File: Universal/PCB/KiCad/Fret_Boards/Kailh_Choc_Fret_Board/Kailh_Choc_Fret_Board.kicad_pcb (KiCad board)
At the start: 2 copper layers, 121 x 29 mm, 24 parts

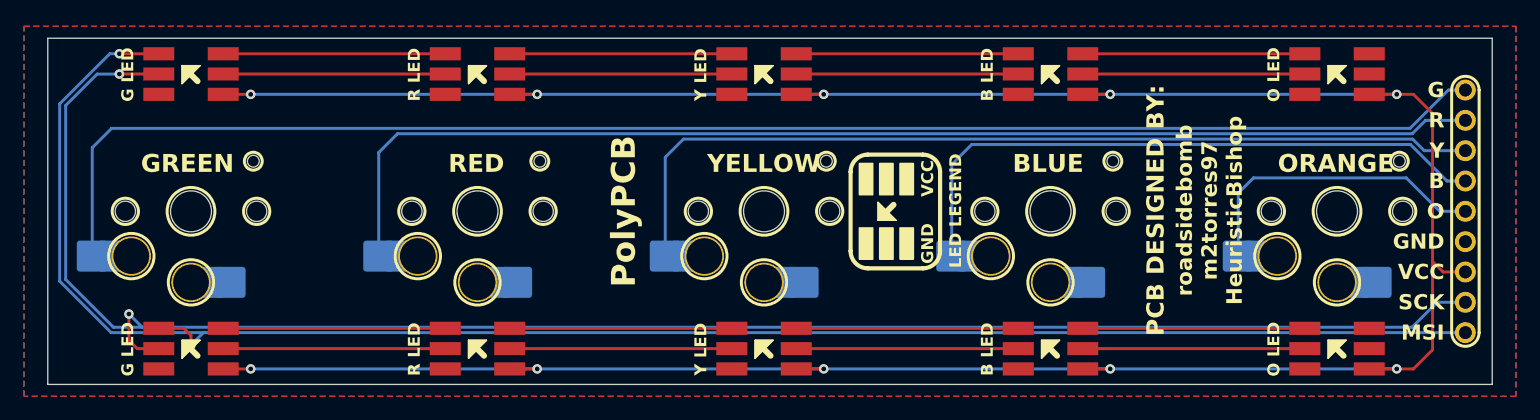
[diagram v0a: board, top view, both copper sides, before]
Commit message: updated The choc fret board
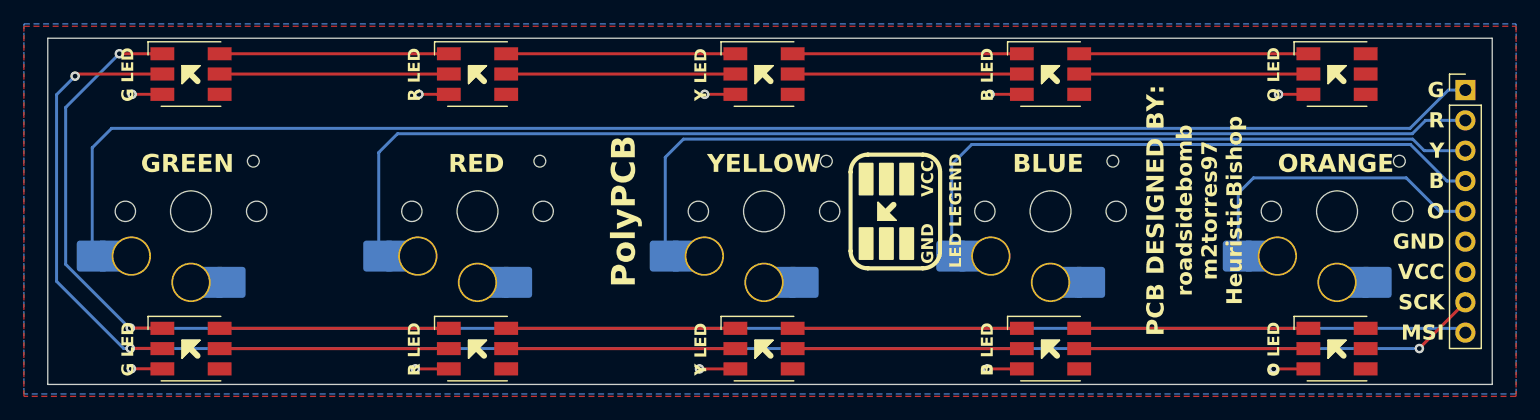
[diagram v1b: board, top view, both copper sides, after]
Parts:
- removed ? (x9): , 
- added J1: Conn_01x09_Pin, Connector_PinHeader_2.54mm:PinHeader_1x09_P2.54mm_Vertical, F.Cu at (180.8, 79.8)
- L1, U1: renamed from D1; footprint Controller_Inputs:LED_RGB_5050_DOTSTAR -> LED_SMD:LED_RGB_5050-6
- L2, U2: renamed from D2; footprint Controller_Inputs:LED_RGB_5050_DOTSTAR -> LED_SMD:LED_RGB_5050-6
- L3, U3: renamed from D3; footprint Controller_Inputs:LED_RGB_5050_DOTSTAR -> LED_SMD:LED_RGB_5050-6
- L4, U4: renamed from D4; footprint Controller_Inputs:LED_RGB_5050_DOTSTAR -> LED_SMD:LED_RGB_5050-6
- L5, U5: renamed from D5; footprint Controller_Inputs:LED_RGB_5050_DOTSTAR -> LED_SMD:LED_RGB_5050-6
- SW1, SW2, SW3, SW4, SW5: renamed from REF**; value Kailh_socket_PG1350 -> SW_HS; footprint Controller_Inputs:Kailh_Hotswap_PG1350 -> Minibar:Kailh_Hotswap_Choc
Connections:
- net led_mosi renamed fret_mosi
- net led_sck renamed fret_sck
- L1 pad 5: Net-(D1-CO) -> Net-(L1-CO)
- L1 pad 6: Net-(D1-DO) -> Net-(L1-DO)
- L2 pad 1: Net-(D1-DO) -> Net-(L1-DO)
- L2 pad 2: Net-(D1-CO) -> Net-(L1-CO)
- L2 pad 5: Net-(D2-CO) -> Net-(L2-CO)
- L2 pad 6: Net-(D2-DO) -> Net-(L2-DO)
- L3 pad 1: Net-(D2-DO) -> Net-(L2-DO)
- L3 pad 2: Net-(D2-CO) -> Net-(L2-CO)
- L3 pad 5: Net-(D3-CO) -> Net-(L3-CO)
- L3 pad 6: Net-(D3-DO) -> Net-(L3-DO)
- L4 pad 1: Net-(D3-DO) -> Net-(L3-DO)
- L4 pad 2: Net-(D3-CO) -> Net-(L3-CO)
- L4 pad 5: Net-(D4-CO) -> Net-(L4-CO)
- L4 pad 6: Net-(D4-DO) -> Net-(L4-DO)
- L5 pad 1: Net-(D4-DO) -> Net-(L4-DO)
- L5 pad 2: Net-(D4-CO) -> Net-(L4-CO)
- L5 pad 5: unconnected-(D5-CO-Pad5) -> unconnected-(L5-CO-Pad5)
- L5 pad 6: unconnected-(D5-DO-Pad6) -> unconnected-(L5-DO-Pad6)
- U1 pad 5: Net-(D1-CO) -> Net-(U1-CO)
- U1 pad 6: Net-(D1-DO) -> Net-(U1-DO)
- U2 pad 1: Net-(D1-DO) -> Net-(U1-DO)
- U2 pad 2: Net-(D1-CO) -> Net-(U1-CO)
- U2 pad 5: Net-(D2-CO) -> Net-(U2-CO)
- U2 pad 6: Net-(D2-DO) -> Net-(U2-DO)
- U3 pad 1: Net-(D2-DO) -> Net-(U2-DO)
- U3 pad 2: Net-(D2-CO) -> Net-(U2-CO)
- U3 pad 5: Net-(D3-CO) -> Net-(U3-CO)
- U3 pad 6: Net-(D3-DO) -> Net-(U3-DO)
- U4 pad 1: Net-(D3-DO) -> Net-(U3-DO)
- U4 pad 2: Net-(D3-CO) -> Net-(U3-CO)
- U4 pad 5: Net-(D4-CO) -> Net-(U4-CO)
- U4 pad 6: Net-(D4-DO) -> Net-(U4-DO)
- U5 pad 1: Net-(D4-DO) -> Net-(U4-DO)
- U5 pad 2: Net-(D4-CO) -> Net-(U4-CO)
- U5 pad 5: unconnected-(D5-CO-Pad5) -> unconnected-(U5-CO-Pad5)
- U5 pad 6: unconnected-(D5-DO-Pad6) -> unconnected-(U5-DO-Pad6)
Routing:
- net VCC: track 245.2 -> 0.00 mm, vias 10 -> 0
- net Net-(D4-DO): track 37.2 -> 0.00 mm
- net Net-(D4-CO): track 37.2 -> 0.00 mm
- net Net-(D3-DO): track 37.2 -> 0.00 mm
- net Net-(D3-CO): track 37.2 -> 0.00 mm
- net Net-(D2-DO): track 37.2 -> 0.00 mm
- net Net-(D2-CO): track 37.2 -> 0.00 mm
- net Net-(D1-DO): track 37.2 -> 0.00 mm
- net Net-(D1-CO): track 37.2 -> 0.00 mm
- net GND: track 0.00 -> 24.0 mm, vias 0 -> 10
- net Net-(U4-DO): track 0.00 -> 18.6 mm
- net Net-(U4-CO): track 0.00 -> 18.6 mm
- net Net-(L4-DO): track 0.00 -> 18.6 mm
- net Net-(L4-CO): track 0.00 -> 18.6 mm
- net Net-(U3-DO): track 0.00 -> 18.6 mm
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- added copper zone on F.Cu, net VCC
- removed copper zone on F.Cu, net GND
